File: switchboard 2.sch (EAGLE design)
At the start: 217 parts, among them IC1 MT8816AP, IC10 Z8F2480SO, IC11 LMV321M5, IC12 74HC595D, IC14 74LVC1G125DBV, IC15 74LVC1G125DBV, IC16 LM2940-9, IC17 PC817S OPTO, IC2 NE5532D, IC3 TC7660-SOIC, IC4 TC7660-SOIC, IC5 FT232RL, IC6 78L05F, IC7 REG1117, IC8 SPI_MEMORY-SOIC, IC9 NE5532D, Q3 FDN352AP, X1 MINI-USB-SCHIELD-32005-301

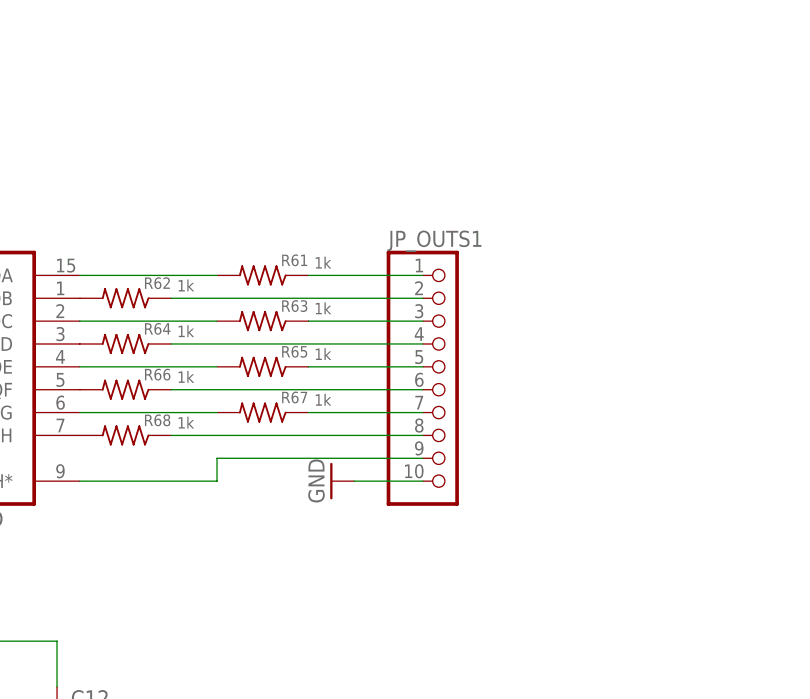
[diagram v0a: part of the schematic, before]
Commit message: Layout development.
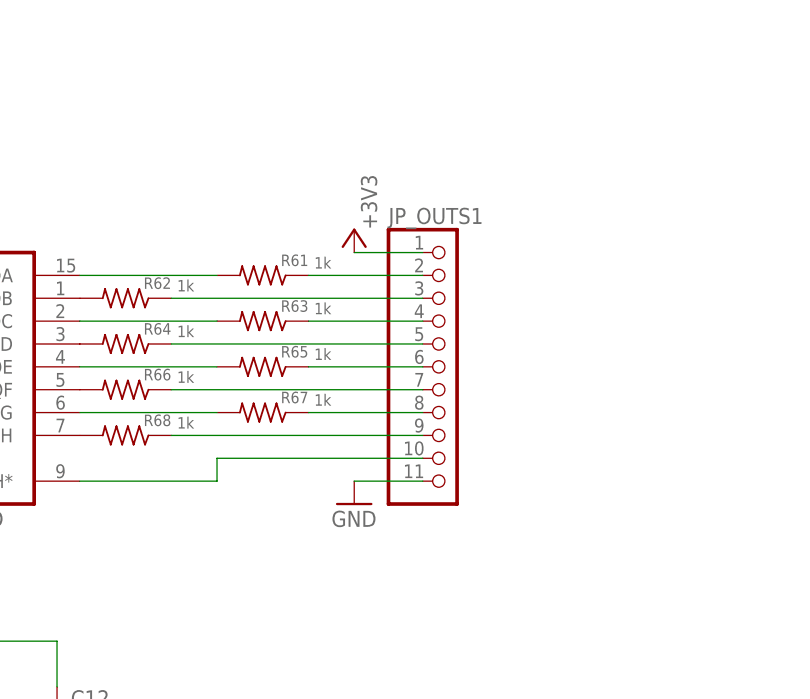
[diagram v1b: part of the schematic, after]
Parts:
- JP_OUTS1: device pinhead:PINHD-1X10 -> pinhead:PINHD-1X11
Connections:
- net +3V3: now also JP_OUTS1.1
- net GND: now also JP_OUTS1.11; no longer JP_OUTS1.10
- net N$36: now also JP_OUTS1.2; no longer JP_OUTS1.1
- net N$37: now also JP_OUTS1.3; no longer JP_OUTS1.2
- net N$38: now also JP_OUTS1.4; no longer JP_OUTS1.3
- net N$39: now also JP_OUTS1.5; no longer JP_OUTS1.4
- net N$40: now also JP_OUTS1.6; no longer JP_OUTS1.5
- net N$41: now also JP_OUTS1.7; no longer JP_OUTS1.6
- net N$42: now also JP_OUTS1.8; no longer JP_OUTS1.7
- net N$43: now also JP_OUTS1.9; no longer JP_OUTS1.8
- net N$44: now also JP_OUTS1.10; no longer JP_OUTS1.9
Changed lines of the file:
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@@
 <part name="D6" library="LUIS" deviceset="SS14" device=""/>
 <part name="GND78" library="supply1" deviceset="GND" device=""/>
-<part name="JP_OUTS1" library="pinhead" deviceset="PINHD-1X10" device=""/>
 <part name="GND81" library="supply1" deviceset="GND" device=""/>
 <part name="GND82" library="supply1" deviceset="GND" device=""/>
@@
 <part name="GND100" library="supply1" deviceset="GND" device=""/>
 <part name="SJ4" library="jumper" deviceset="SJ" device=""/>
+<part name="JP_OUTS1" library="pinhead" library_urn="urn:adsk.eagle:library:325" deviceset="PINHD-1X11" device="" package3d_urn="urn:adsk.eagle:package:22410/1"/>
+<part name="U$2" library="supply1" deviceset="+3V3" device=""/>
 </parts>
 <sheets>
@@
 <instance part="D6" gate="G$1" x="60.96" y="228.6" rot="MR0"/>
 <instance part="GND78" gate="1" x="101.6" y="-48.26" rot="MR0"/>
-<instance part="JP_OUTS1" gate="A" x="393.7" y="45.72"/>
-<instance part="GND81" gate="1" x="381" y="33.02" rot="R270"/>
+<instance part="GND81" gate="1" x="383.54" y="30.48"/>
 <instance part="GND82" gate="1" x="-38.1" y="-370.84"/>
 <instance part="IC12" gate="P" x="340.36" y="7.62"/>
@@
 <instance part="GND100" gate="1" x="96.52" y="-294.64"/>
 <instance part="SJ4" gate="1" x="-365.76" y="91.44" rot="MR0"/>
+<instance part="JP_OUTS1" gate="A" x="393.7" y="45.72"/>
+<instance part="U$2" gate="G$1" x="383.54" y="60.96" smashed="yes">
+<attribute name="VALUE" x="386.08" y="60.96" size="1.778" layer="96" rot="R90"/>
+</instance>
 </instances>
 <busses>
@@
 <wire x1="-370.84" y1="91.44" x2="-375.92" y2="91.44" width="0.1524" layer="91"/>
 </segment>
+<segment>
+<pinref part="JP_OUTS1" gate="A" pin="1"/>
+<pinref part="U$2" gate="G$1" pin="+3V3"/>
+<wire x1="383.54" y1="58.42" x2="391.16" y2="58.42" width="0.1524" layer="91"/>
+</segment>
 </net>
 <net name="GND" class="0">
@@
 <segment>
 <pinref part="GND81" gate="1" pin="GND"/>
-<pinref part="JP_OUTS1" gate="A" pin="10"/>
 <wire x1="383.54" y1="33.02" x2="391.16" y2="33.02" width="0.1524" layer="91"/>
+<pinref part="JP_OUTS1" gate="A" pin="11"/>
 </segment>
 <segment>
@@
 <segment>
 <pinref part="R61" gate="G$1" pin="1"/>
-<pinref part="JP_OUTS1" gate="A" pin="1"/>
 <wire x1="378.46" y1="55.88" x2="391.16" y2="55.88" width="0.1524" layer="91"/>
+<pinref part="JP_OUTS1" gate="A" pin="2"/>
 </segment>
 </net>
 <net name="N$37" class="0">
 <segment>
-<pinref part="JP_OUTS1" gate="A" pin="2"/>
 <pinref part="R62" gate="G$1" pin="1"/>
 <wire x1="391.16" y1="53.34" x2="363.22" y2="53.34" width="0.1524" layer="91"/>
+<pinref part="JP_OUTS1" gate="A" pin="3"/>
 </segment>
 </net>
@@
 <segment>
 <pinref part="R63" gate="G$1" pin="1"/>
-<pinref part="JP_OUTS1" gate="A" pin="3"/>
 <wire x1="378.46" y1="50.8" x2="391.16" y2="50.8" width="0.1524" layer="91"/>
+<pinref part="JP_OUTS1" gate="A" pin="4"/>
 </segment>
 </net>
 <net name="N$39" class="0">
 <segment>
-<pinref part="JP_OUTS1" gate="A" pin="4"/>
 <pinref part="R64" gate="G$1" pin="1"/>
 <wire x1="391.16" y1="48.26" x2="363.22" y2="48.26" width="0.1524" layer="91"/>
+<pinref part="JP_OUTS1" gate="A" pin="5"/>
 </segment>
 </net>
@@
 <segment>
 <pinref part="R65" gate="G$1" pin="1"/>
-<pinref part="JP_OUTS1" gate="A" pin="5"/>
 <wire x1="378.46" y1="45.72" x2="391.16" y2="45.72" width="0.1524" layer="91"/>
+<pinref part="JP_OUTS1" gate="A" pin="6"/>
 </segment>
 </net>
 <net name="N$41" class="0">
 <segment>
-<pinref part="JP_OUTS1" gate="A" pin="6"/>
 <pinref part="R66" gate="G$1" pin="1"/>
 <wire x1="391.16" y1="43.18" x2="363.22" y2="43.18" width="0.1524" layer="91"/>
+<pinref part="JP_OUTS1" gate="A" pin="7"/>
 </segment>
 </net>
@@
 <segment>
 <pinref part="R67" gate="G$1" pin="1"/>
-<pinref part="JP_OUTS1" gate="A" pin="7"/>
 <wire x1="378.46" y1="40.64" x2="391.16" y2="40.64" width="0.1524" layer="91"/>
+<pinref part="JP_OUTS1" gate="A" pin="8"/>
 </segment>
 </net>
 <net name="N$43" class="0">
 <segment>
-<pinref part="JP_OUTS1" gate="A" pin="8"/>
 <pinref part="R68" gate="G$1" pin="1"/>
 <wire x1="391.16" y1="38.1" x2="363.22" y2="38.1" width="0.1524" layer="91"/>
+<pinref part="JP_OUTS1" gate="A" pin="9"/>
 </segment>
 </net>
@@
 <net name="N$44" class="0">
 <segment>
-<pinref part="JP_OUTS1" gate="A" pin="9"/>
 <wire x1="391.16" y1="35.56" x2="368.3" y2="35.56" width="0.1524" layer="91"/>
 <wire x1="368.3" y1="35.56" x2="368.3" y2="33.02" width="0.1524" layer="91"/>
 <pinref part="IC12" gate="A" pin="QH*"/>
 <wire x1="368.3" y1="33.02" x2="353.06" y2="33.02" width="0.1524" layer="91"/>
+<pinref part="JP_OUTS1" gate="A" pin="10"/>
 </segment>
 </net>
@@
 will not be understood (or retained) with this version.
 </note>
+<note version="8.3" severity="warning">
+Since Version 8.3, EAGLE supports the association of 3D packages
+with devices in libraries, schematics, and board files. Those 3D
+packages will not be understood (or retained) with this version.
+</note>
 </compatibility>
